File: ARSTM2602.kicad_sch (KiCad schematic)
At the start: 0 parts

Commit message: aaa
gitdesktop test
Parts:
- added U1: STM32H523CCTx, Package_QFP:LQFP-48_7x7mm_P0.5mm, symbol MCU_ST_STM32H5:STM32H523CCTx
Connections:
- new net: U1.23 (VSS), U1.35 (VSS), U1.47 (VSS)
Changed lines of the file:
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@@
 (kicad_sch
-	(version 20250114)
+	(version 20260306)
 	(generator "eeschema")
-	(generator_version "9.0")
+	(generator_version "10.0")
 	(paper "A4")
-	(sheet_instances
-		(path "/"
-			(page "1")
-		)
-	)
-	(embedded_fonts no)
-)

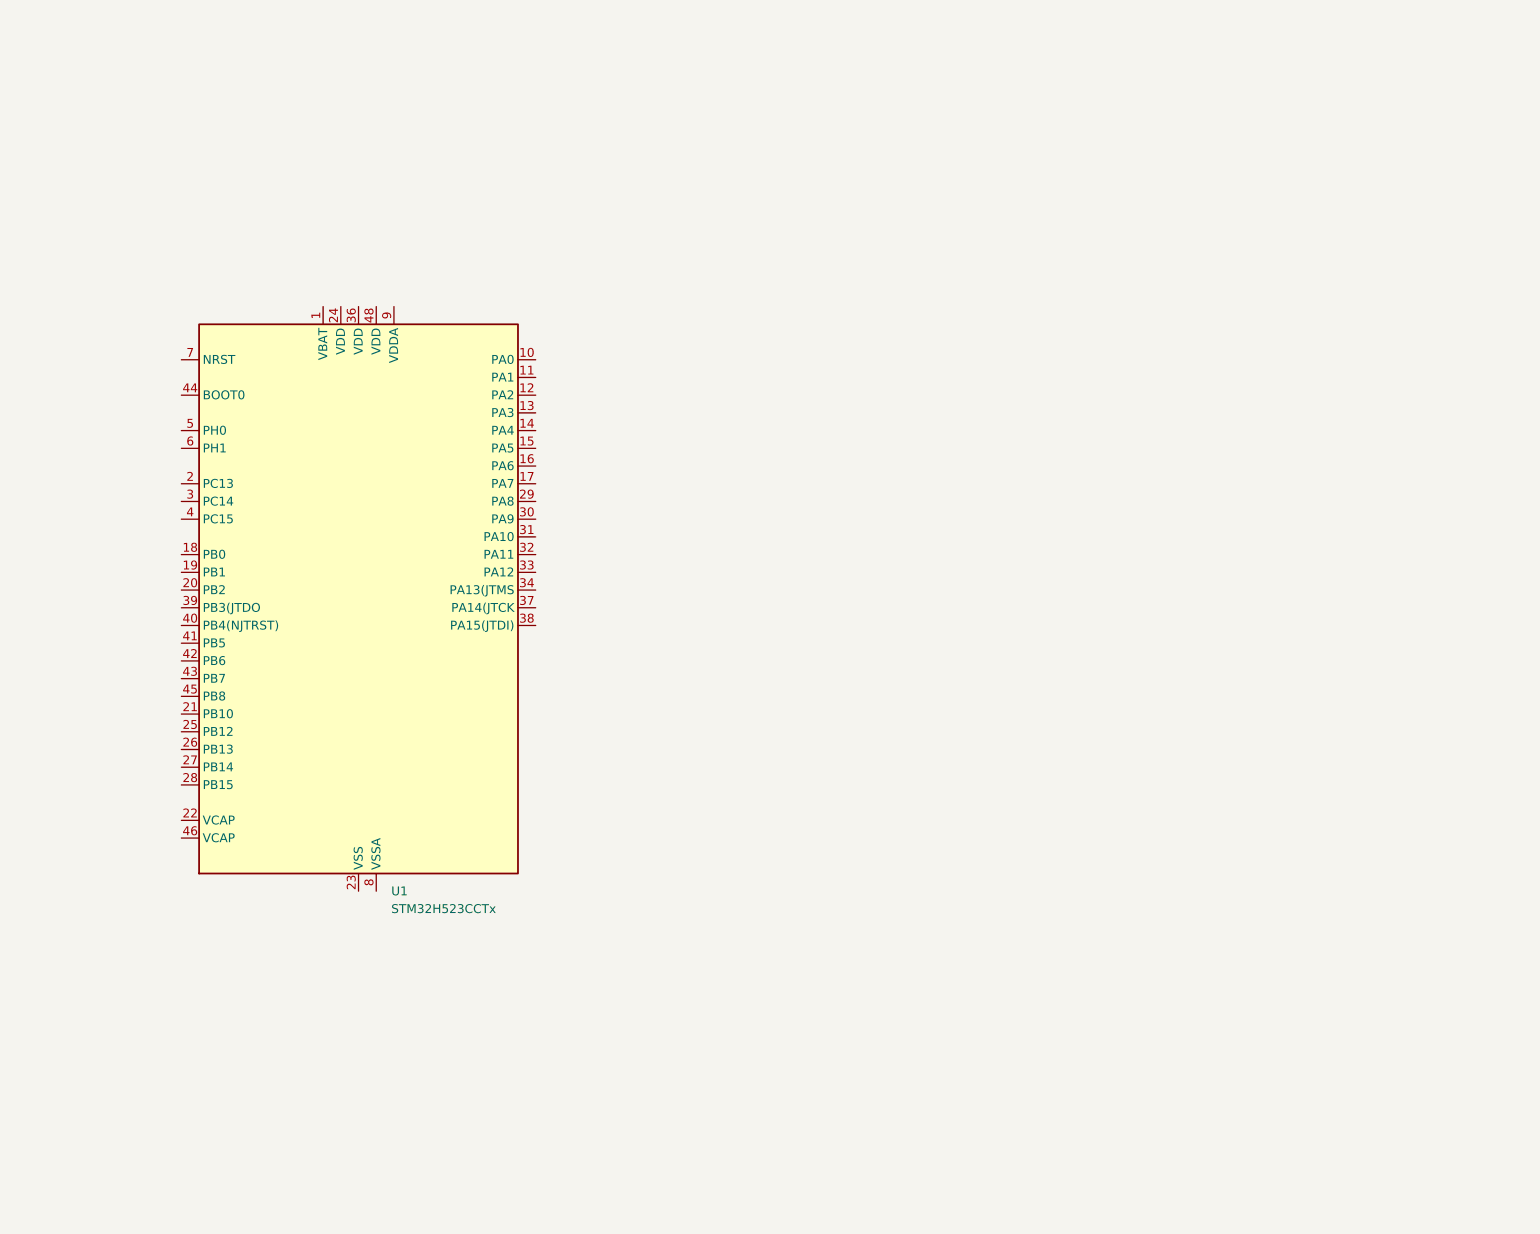
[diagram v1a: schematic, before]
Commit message: 回路図をこぴった
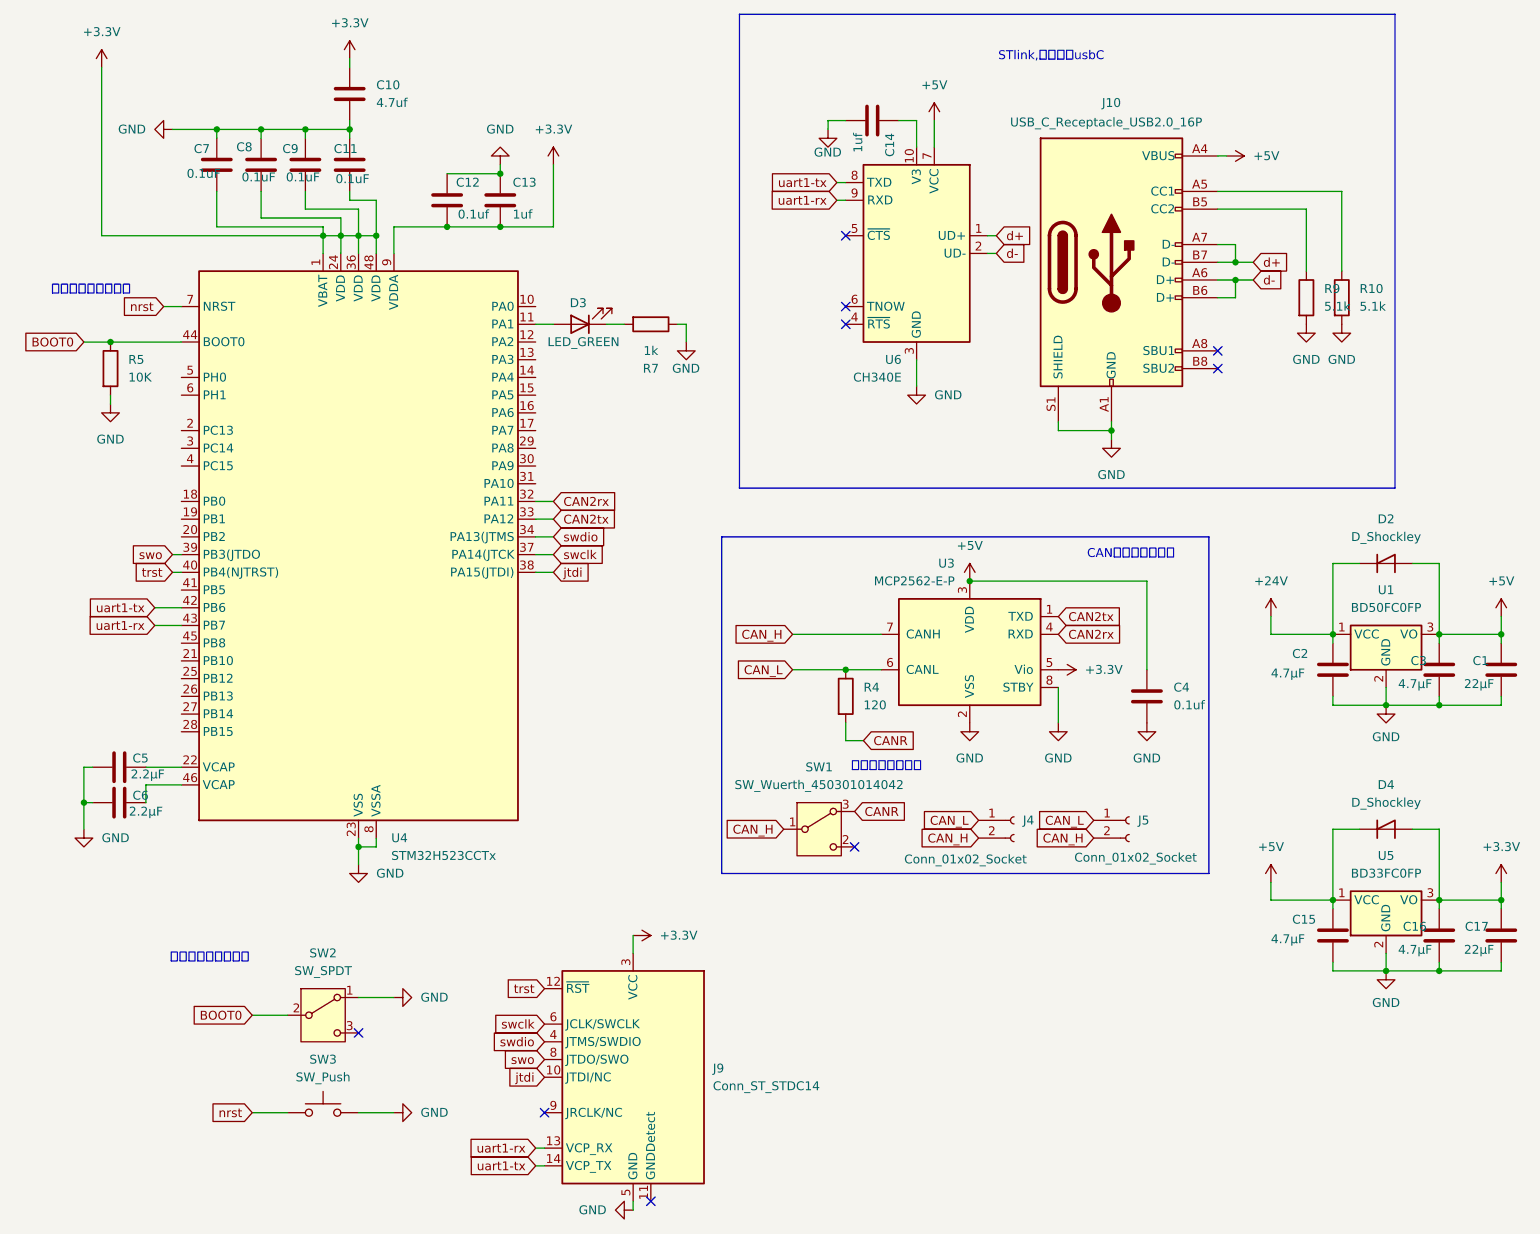
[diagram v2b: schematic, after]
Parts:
- removed U1: STM32H523CCTx, Package_QFP:LQFP-48_7x7mm_P0.5mm, symbol MCU_ST_STM32H5:STM32H523CCTx
- added C1, C17: 22μF, Capacitor_SMD:C_0805_2012Metric_Pad1.18x1.45mm_HandSolder, symbol Device:C
- added C10: 4.7uf, Capacitor_SMD:C_0805_2012Metric_Pad1.18x1.45mm_HandSolder, symbol Device:C
- added C11, C7, C8, C9: 0.1uF, Capacitor_SMD:C_0603_1608Metric_Pad1.08x0.95mm_HandSolder, symbol Device:C
- added C12, C4: 0.1uf, Capacitor_SMD:C_0603_1608Metric_Pad1.08x0.95mm_HandSolder, symbol Device:C
- added C13, C14: 1uf, Capacitor_SMD:C_0603_1608Metric_Pad1.08x0.95mm_HandSolder, symbol Device:C
- added C15, C16, C2, C3: 4.7μF, Capacitor_SMD:C_0805_2012Metric_Pad1.18x1.45mm_HandSolder, symbol Device:C
- added C5, C6: 2.2μF, Capacitor_SMD:C_0603_1608Metric_Pad1.08x0.95mm_HandSolder, symbol Device:C
- added D2, D4: D_Shockley, Diode_SMD:D_SOD-323_HandSoldering, symbol Device:D_Shockley
- added D3: LED_GREEN, Capacitor_SMD:C_0603_1608Metric_Pad1.08x0.95mm_HandSolder, symbol Device:LED
- added J10: USB_C_Receptacle_USB2.0_16P, Connector_USB:USB_C_Receptacle_GCT_USB4105-xx-A_16P_TopMnt_Horizontal, symbol Connector:USB_C_Receptacle_USB2.0_16P
- added J4, J5: Conn_01x02_Socket, Connector_JST:JST_XH_S2B-XH-A-1_1x02_P2.50mm_Horizontal, symbol Connector:Conn_01x02_Socket
- added J9: Conn_ST_STDC14, Connector_PinHeader_1.27mm:PinHeader_2x07_P1.27mm_Vertical, symbol Connector:Conn_ST_STDC14
- added R10, R9: 5.1k, Resistor_SMD:R_0603_1608Metric_Pad0.98x0.95mm_HandSolder, symbol Device:R
- added R4: 120, Resistor_SMD:R_0603_1608Metric_Pad0.98x0.95mm_HandSolder, symbol Device:R
- added R5: 10K, Resistor_SMD:R_0603_1608Metric_Pad0.98x0.95mm_HandSolder, symbol Device:R
- added R7: 1k, Resistor_SMD:R_0603_1608Metric_Pad0.98x0.95mm_HandSolder, symbol Device:R
- added SW1: SW_Wuerth_450301014042, Button_Switch_THT:SW_Slide-03_Wuerth-WS-SLTV_10x2.5x6.4_P2.54mm, symbol Switch:SW_Wuerth_450301014042
- added SW2: SW_SPDT, Button_Switch_THT:SW_Slide-03_Wuerth-WS-SLTV_10x2.5x6.4_P2.54mm, symbol Switch:SW_SPDT
- added SW3: SW_Push, Button_Switch_THT:SW_PUSH_6mm, symbol Switch:SW_Push
- added U1: BD50FC0FP, Package_TO_SOT_SMD:TO-252-2, symbol Regulator_Linear:BD50FC0FP
- added U3: MCP2562-E-P, Package_DIP:DIP-8_W7.62mm, symbol Interface_CAN_LIN:MCP2562-E-P
- added U4: STM32H523CCTx, Package_QFP:LQFP-48_7x7mm_P0.5mm, symbol MCU_ST_STM32H5:STM32H523CCTx
- added U5: BD33FC0FP, Package_TO_SOT_SMD:TO-252-2, symbol Regulator_Linear:BD33FC0FP
- added U6: CH340E, Package_SO:MSOP-10_3x3mm_P0.5mm, symbol Interface_USB:CH340E
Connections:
- new net: D3.1 (K), R7.2
- new net: C6.2, U4.46 (VCAP)
- new net: C5.2, U4.22 (VCAP)
- new net: J10.A5 (CC1), R10.1
- new net: J10.B5 (CC2), R9.1
- new net: D3.2 (A), U4.11 (PA1)
- new net: C14.1, U6.10 (V3)
- new net +24V: C2.1, D2.1 (K), U1.1 (VCC)
- new net +3.3V: C10.1, C11.1, C12.2, C13.2, C16.1, C17.1, C7.1, C8.1, C9.1, D4.2 (A), J9.3 (VCC), U3.5 (Vio), U4.1 (VBAT), U4.24 (VDD), U4.36 (VDD), U4.48 (VDD), U4.9 (VDDA), U5.3 (VO)
- new net +5V: C1.1, C15.1, C3.1, C4.1, D2.2 (A), D4.1 (K), J10.A4 (VBUS), J10.A9 (VBUS), J10.B4 (VBUS), J10.B9 (VBUS), U1.3 (VO), U3.3 (VDD), U5.1 (VCC), U6.7 (VCC)
- new net BOOT0: R5.1, SW2.2 (B), U4.44 (BOOT0)
- new net CAN2rx: U3.4 (RXD), U4.32 (PA11)
- new net CAN2tx: U3.1 (TXD), U4.33 (PA12)
- new net CANR: R4.2, SW1.3 (A)
- new net CAN_H: J4.2 (Pin_2), J5.2 (Pin_2), SW1.1 (B), U3.7 (CANH)
- new net CAN_L: J4.1 (Pin_1), J5.1 (Pin_1), R4.1, U3.6 (CANL)
- new net GND: C1.2, C10.2, C11.2, C12.1, C13.1, C14.2, C15.2, C16.2, C17.2, C2.2, C3.2, C4.2, C5.1, C6.1, C7.2, C8.2, C9.2, J10.A1 (GND), J10.A12 (GND), J10.B1 (GND), J10.B12 (GND), J10.S1 (SHIELD), J9.5 (GND), J9.7 (GND), R10.2, R5.2, R7.1, R9.2, SW2.1 (A), SW3.2, U1.2 (GND), U3.2 (VSS), U3.8 (STBY), U4.23 (VSS), U4.35 (VSS), U4.47 (VSS), U4.8 (VSSA), U5.2 (GND), U6.3 (GND)
- new net d+: J10.A7 (D-), J10.B7 (D-), U6.1 (UD+)
- new net d-: J10.A6 (D+), J10.B6 (D+), U6.2 (UD-)
- new net jtdi: J9.10 (JTDI/NC), U4.38 (PA15(JTDI))
- new net nrst: SW3.1, U4.7 (NRST)
- new net swclk: J9.6 (JCLK/SWCLK), U4.37 (PA14(JTCK)
- new net swdio: J9.4 (JTMS/SWDIO), U4.34 (PA13(JTMS)
- new net swo: J9.8 (JTDO/SWO), U4.39 (PB3(JTDO)
- new net trst: J9.12 (~{RST}), U4.40 (PB4(NJTRST))
- new net uart1-rx: J9.13 (VCP_RX), U4.43 (PB7), U6.9 (RXD)
- new net uart1-tx: J9.14 (VCP_TX), U4.42 (PB6), U6.8 (TXD)
- no-connect marks 0 -> 9
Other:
- note added: "CANトランシーバー"
- note added: "STlink,電源供給usbC"
- note added: "リセット用スイッチ"
- note added: "終端抵抗オンオフ"
